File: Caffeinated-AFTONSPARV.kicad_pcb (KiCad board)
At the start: 4 copper layers, 42.5 x 16.1 mm, 35 parts, among them J1 Conn_01x02, J2 Conn_01x04, J3 TagConnect, Q1 AO3400A, Q2 AO3400A, Q3 AO3400A, SW1 SW_Push, U1 ESP32-C3-MINI-1, U2 SY8201ABC

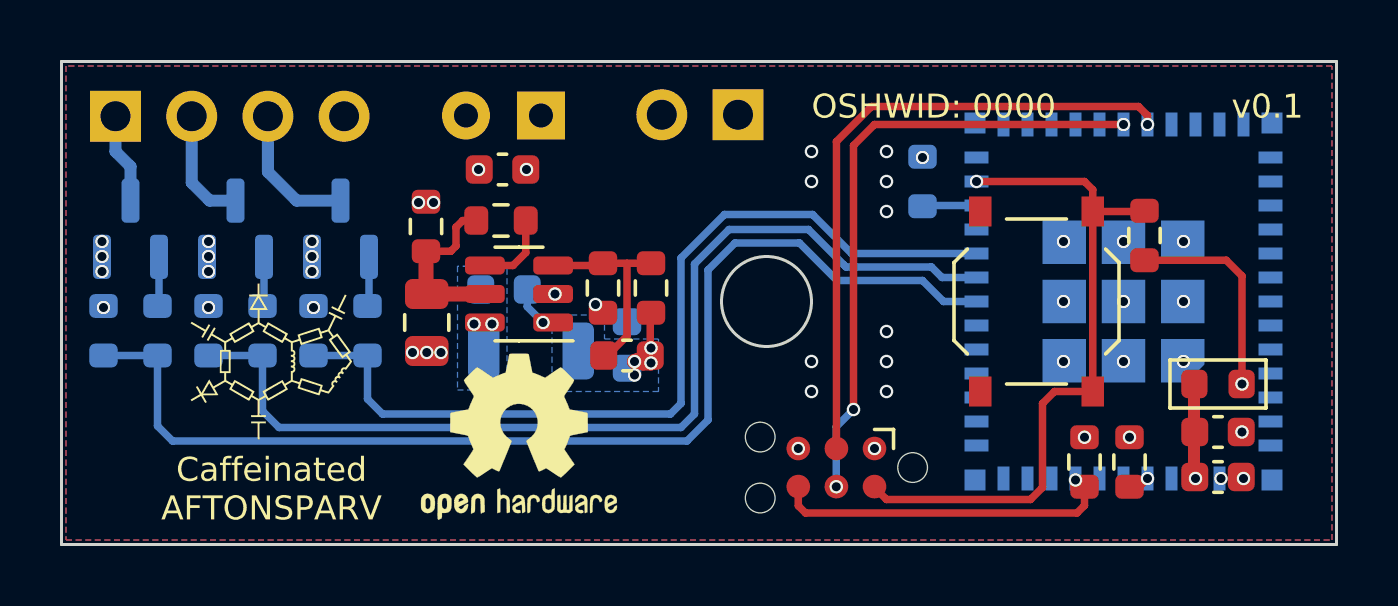
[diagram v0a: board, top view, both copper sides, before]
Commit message: feat(): Rework and finalize design
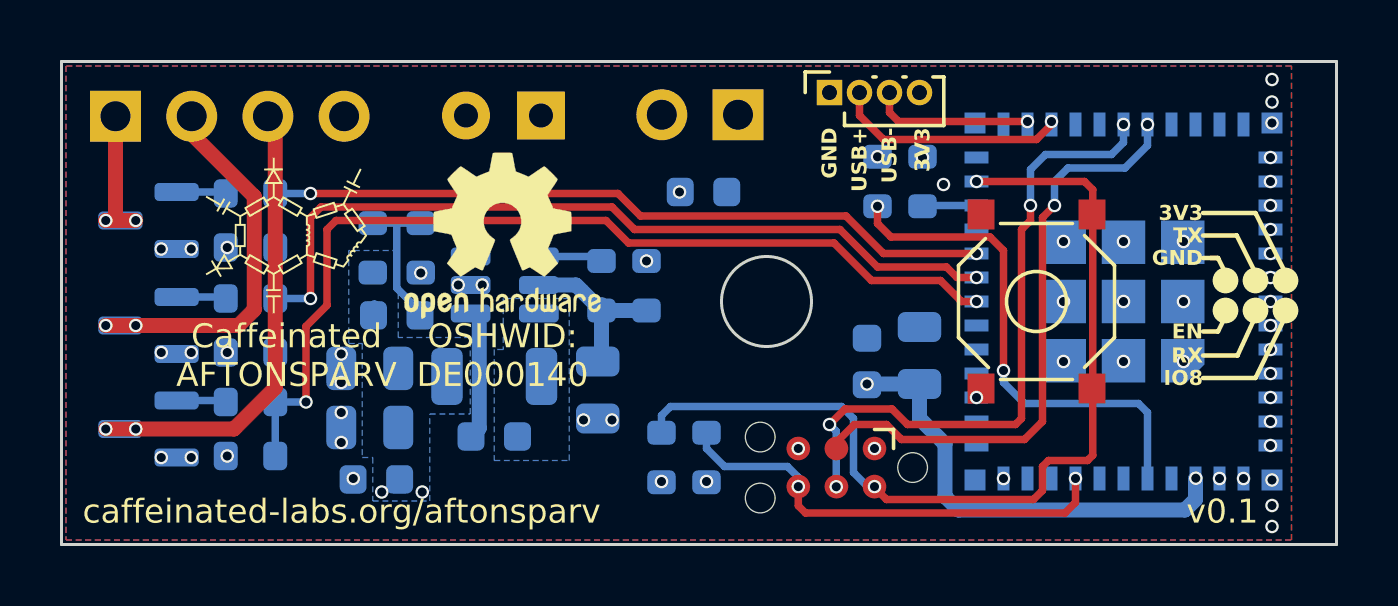
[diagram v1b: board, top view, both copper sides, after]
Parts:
- removed C8: 100uF, Capacitor_SMD:C_0603_1608Metric
- removed FB1: FerriteBead, PCM_Ferrite_SMD_AKL:Ferrite_0603_1608Metric
- added C10: 4.7uF, Capacitor_SMD:C_0805_2012Metric, B.Cu at (140.1, 104.2)
- added C11: 100nF, Capacitor_SMD:C_0603_1608Metric, B.Cu at (140.3, 105.9)
- added C9: 4.7uF, Capacitor_SMD:C_0805_2012Metric, B.Cu at (140.1, 102.2)
- added J4: USB, Connector_PinSocket_1.00mm:PinSocket_1x04_P1.00mm_Vertical, F.Cu at (155.4, 93.0)
- C1, C3, C5, C7, U2: moved to B.Cu
- C6: value 22uF -> 4.7uF; footprint Capacitor_SMD:C_0603_1608Metric -> Capacitor_SMD:C_0805_2012Metric
- J1: value Conn_01x02 -> PWR
- J2: value Conn_01x04 -> LED
- R1, R2, R3, R9: value 10k -> 10kΩ
- R10, R14, R7, R8: value 10k -> 10kΩ; moved to B.Cu
- R11: value 1 -> 1Ω; moved to B.Cu
- R12: value 100k -> 100kΩ; moved to B.Cu
- R13: value 22,1k -> 22.1kΩ; moved to B.Cu
- R4, R5, R6: value 470 -> 20Ω
- SW1: footprint Button_Switch_SMD:SW_Push_1P1T_XKB_TS-1187A -> caffeinated-labs:YTS-C005
- U1: value ESP32-C3-MINI-1 -> ESP32-C3-MINI-1-[H/N]4
- moved R7 17.7 mm to (149.8, 105.2)
- moved R10 12.6 mm to (151.3, 105.2), turned to 90 degrees
- moved R8 12.6 mm to (157.0, 96.0)
- moved C7 11.9 mm to (156.7, 102.0), turned to 90 degrees
- moved C6 9.76 mm to (158.4, 101.8), turned to 90 degrees
- moved R12 9.37 mm to (140.2, 98.2)
- moved Q1 9.25 mm to (132.7, 104.2), turned to 180 degrees
- moved C5 7.79 mm to (141.0, 100.5), turned to 180 degrees
- moved R11 7.61 mm to (149.3, 99.5)
- moved C1 6.74 mm to (151.2, 96.3), turned to 0 degrees
- moved REF** 6.72 mm to (144.5, 97.8)
- moved R13 6.22 mm to (141.8, 98.2)
- moved C3 6.13 mm to (147.7, 103.0)
- moved R1 5.63 mm to (136.1, 98.2), turned to 180 degrees
- moved R5 5.53 mm to (136.1, 96.4), turned to 180 degrees
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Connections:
- net Net-(J3-EN) renamed EN
- net Net-(J3-IO0/IO8) renamed IO9
- net Net-(J3-RX) renamed RX
- net Net-(J3-TX) renamed TX
- net Net-(U1-GPIO5/ADC2_CH0) renamed LED-G
- C6 pad 1: GND -> +3.3V
- C6 pad 2: +3.3V -> GND
- C7 pad 1: Net-(U1-3V3) -> +3.3V
- R1 pad 1: Net-(U1-GPIO4/ADC1_CH4) -> LED-B
- R3 pad 1: Net-(U1-GPIO6) -> LED-R
- R5 pad 1: Net-(U1-GPIO4/ADC1_CH4) -> LED-B
- R6 pad 1: Net-(U1-GPIO6) -> LED-R
- U1 pad 18: Net-(U1-GPIO4/ADC1_CH4) -> LED-R
- U1 pad 20: Net-(U1-GPIO6) -> LED-B
- U1 pad 26: unconnected-(U1-GPIO18/USB_D--Pad26) -> USB-D-
- U1 pad 27: unconnected-(U1-GPIO19/USB_D+-Pad27) -> USB-D+
- U1 pad 3: Net-(U1-3V3) -> +3.3V
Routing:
- net Net-(U1-GPIO4/ADC1_CH4): track 38.1 -> 0.00 mm
- net LED-R: track 0.00 -> 31.8 mm, vias 0 -> 2
- net Net-(U1-GPIO6): track 29.9 -> 0.00 mm
- net LED-B: track 0.00 -> 26.0 mm, vias 0 -> 2
- net Net-(U1-GPIO2/ADC1_CH2): track 0.71 -> 17.0 mm, vias 1 -> 2
- net Net-(J2-Pin_3): track 4.67 -> 15.4 mm, vias 0 -> 2
- net Net-(J2-Pin_2): track 3.92 -> 12.5 mm, vias 0 -> 2
- net IO9: track 23.1 -> 31.3 mm, vias 1 -> 2
- net USB-D+: track 0.00 -> 7.80 mm, vias 0 -> 1
- net USB-D-: track 0.00 -> 5.39 mm, vias 0 -> 1
- net LED-G: track 34.0 -> 29.0 mm, vias 0 -> 2
- net +3.3V: track 10.4 -> 15.1 mm
- net EN: track 11.0 -> 15.2 mm, vias 1 -> 2
- net Net-(U1-3V3): track 3.19 -> 0.00 mm, vias 1 -> 0
- net Net-(U2-BS): track 1.32 -> 4.50 mm, vias 1 -> 0
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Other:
- board text added: "3V3"
- board text added: "EN"
- board text added: "GND"
- board text added: "IO8"
- board text added: "OSHWID: DE000140"
- board text added: "RX"
- board text added: "TX"
- board text added: "USB+"
- board text added: "USB-"
- board text removed: "OSHWID: 0000"
